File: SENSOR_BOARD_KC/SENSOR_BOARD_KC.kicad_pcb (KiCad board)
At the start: 2 copper layers, 199 x 120 mm, 34 parts, among them SW2 SW_Push, SW3 SW_Push, SW4 SW_Push, SW5 SW_Push, U1 BP

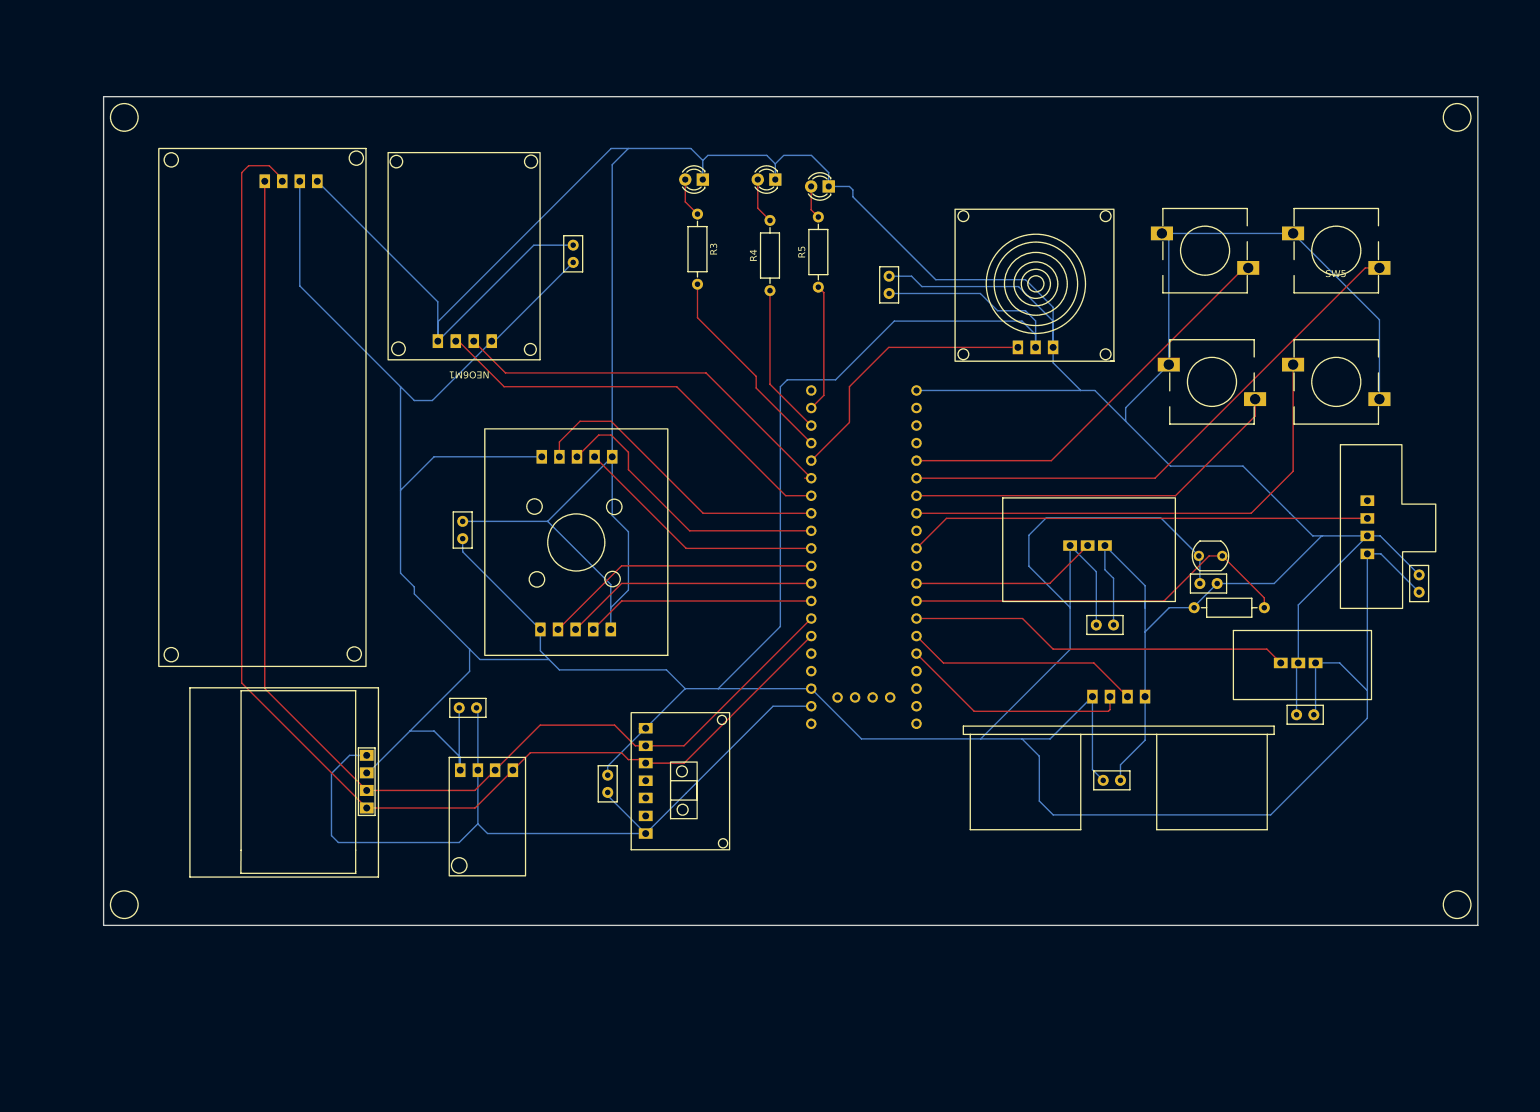
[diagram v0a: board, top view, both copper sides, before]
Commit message: Some changes in pcb
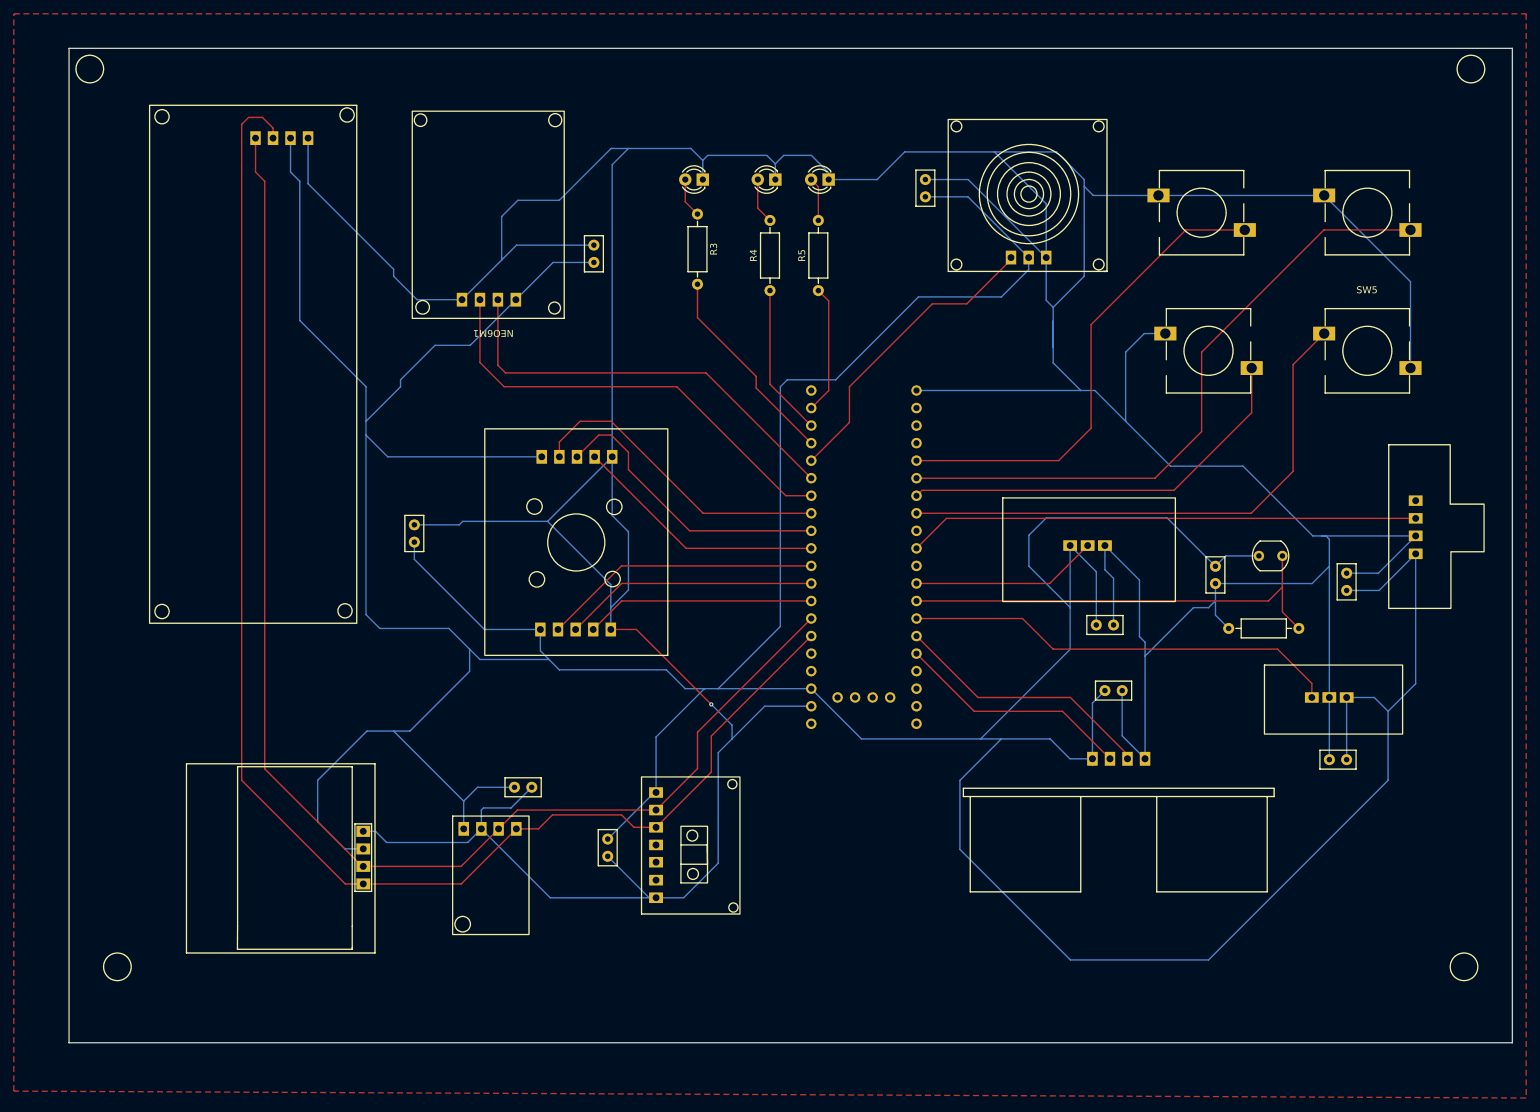
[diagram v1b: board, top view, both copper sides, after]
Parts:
- moved C7 15.0 mm to (186.0, 51.5)
- moved C12 14.0 mm to (126.5, 137.0)
- moved TTP1 13.0 mm to (201.0, 51.0)
- moved C2 13.0 mm to (212.0, 123.0)
- moved OLED1 11.0 mm to (94.0, 147.0)
- moved C5 10.5 mm to (247.0, 108.5)
- moved MAX1 9.42 mm to (152.0, 146.0)
- moved C11 9.25 mm to (140.0, 144.5)
- moved Ultrasonic1 9.00 mm to (214.0, 132.9)
- moved R2 8.70 mm to (234.3, 103.5)
- moved BMP1 8.51 mm to (123.0, 150.0)
- moved C1 8.05 mm to (247.0, 133.0)
- moved SW3 7.11 mm to (250.0, 54.0)
- moved C8 7.02 mm to (112.0, 101.5)
- moved MQ1 7.00 mm to (257.3, 99.2)
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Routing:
- net Net-(BMP1-vcc): track 654.1 -> 767.6 mm
- net Net-(BMP1-gnd): track 728.5 -> 814.9 mm, vias 0 -> 1
- net Net-(BMP1-SDA): track 182.9 -> 210.5 mm
- net Net-(BMP1-SCL): track 171.5 -> 194.9 mm
- net Net-(SW3-Pad2): track 79.6 -> 93.2 mm
- net Net-(SW2-Pad2): track 59.6 -> 70.2 mm
- net Net-(R1-Pad1): track 57.0 -> 65.3 mm
- net Net-(SW1-d0): track 55.4 -> 63.2 mm
- net Net-(MQ1-d0): track 67.1 -> 74.1 mm
- net Net-(SW5-Pad1): track 72.5 -> 78.9 mm
- net Net-(TTP1-Data): track 39.8 -> 44.3 mm
- net Net-(NEO6M1-TX): track 60.7 -> 65.1 mm
- net Net-(Ultrasonic1-echo): track 34.2 -> 38.3 mm
- net Net-(SW4-Pad2): track 56.3 -> 60.0 mm
- net Net-(NEO6M1-RX): track 58.1 -> 61.6 mm
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- added copper zone on F.Cu, net (none)
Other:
- board size 199 x 120 mm -> 209 x 144 mm
